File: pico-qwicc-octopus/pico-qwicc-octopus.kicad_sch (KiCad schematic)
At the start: 21 parts, among them U1 RP2040

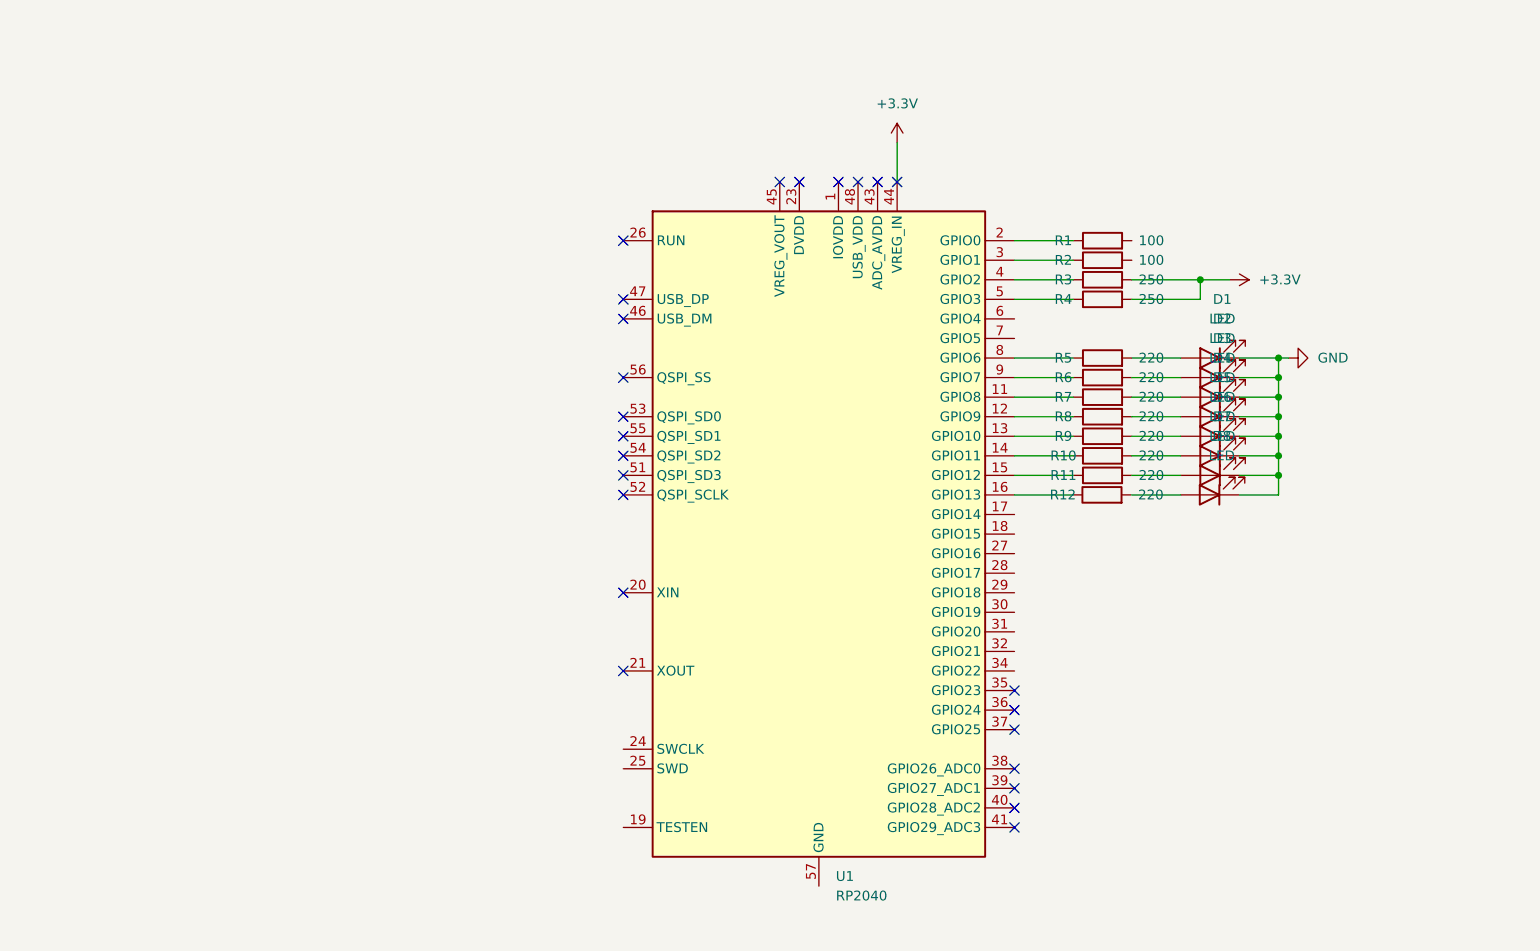
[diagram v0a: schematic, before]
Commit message: Trying to get just the basics working.
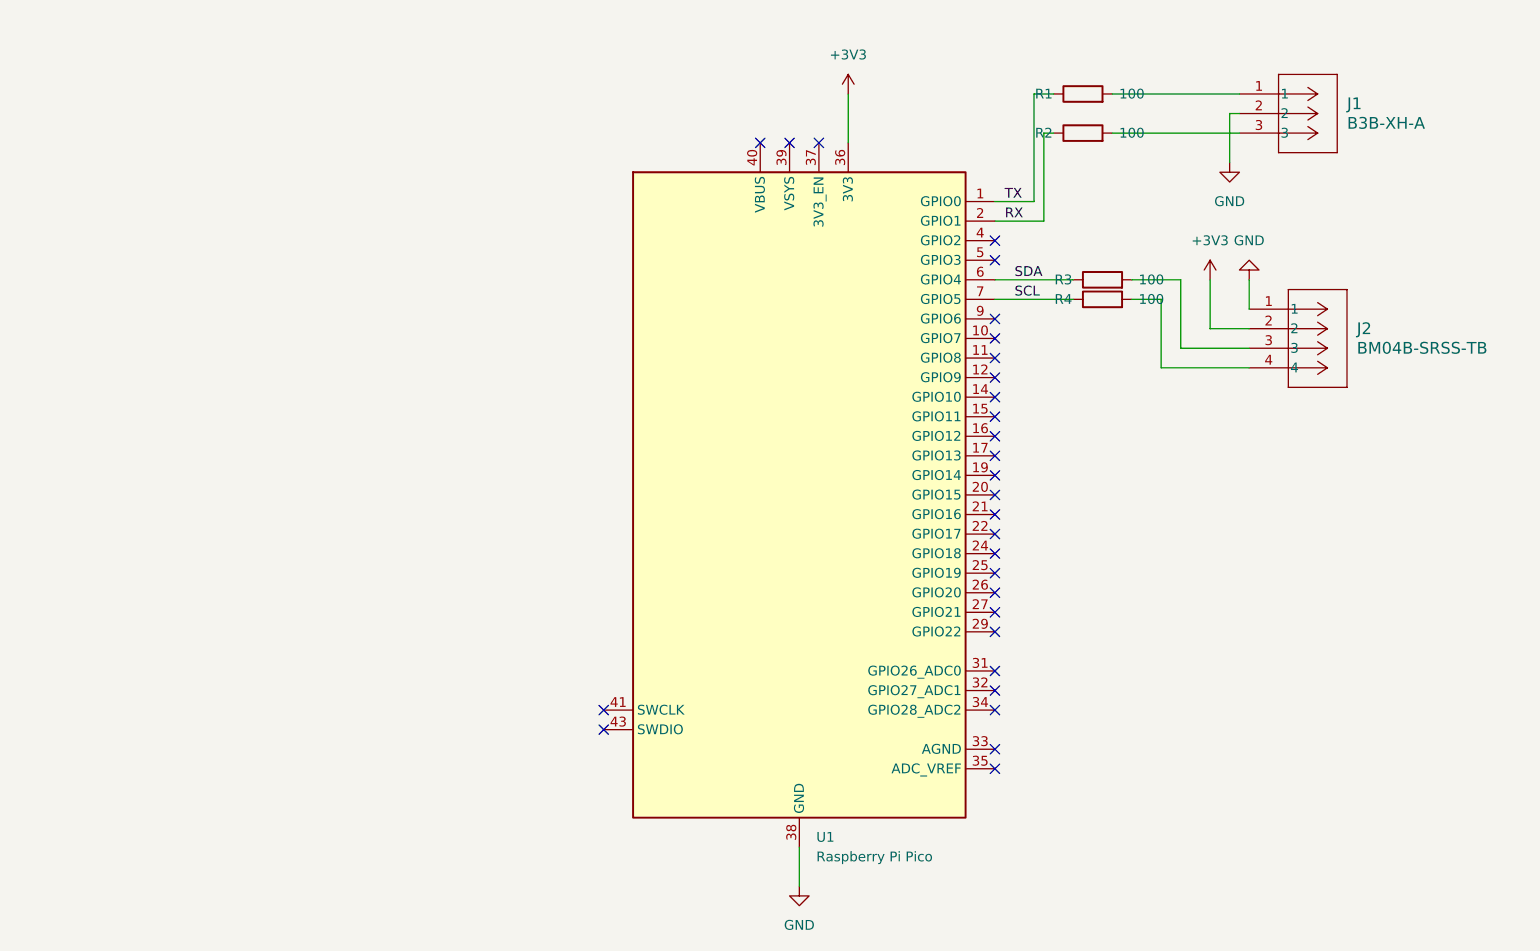
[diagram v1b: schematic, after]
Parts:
- removed D1, D2, D3, D4, D6, D7, D8: LED, LED_SMD:LED_0805_2012Metric, symbol Device:LED
- removed D5: LED, symbol Device:LED
- removed R10, R11, R12, R5, R6, R7, R8, R9: 220, Resistor_SMD:R_0805_2012Metric, symbol Device:R
- removed U1: RP2040, Package_DFN_QFN:QFN-56-1EP_7x7mm_P0.4mm_EP3.2x3.2mm, symbol MCU_RaspberryPi:RP2040
- added J1: B3B-XH-A, CONN_B3B-XH-A_JST, symbol Ivan Hawkes:B3B-XH-A
- added J2: BM04B-SRSS-TB, CONN4_BM04B-SRSS_JST, symbol Ivan Hawkes:BM04B-SRSS-TB
- added U1: Raspberry Pi Pico, Footprint, symbol Ivan Hawkes:Raspberry_Pi_Pico
- R3, R4: value 250 -> 100
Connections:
- net GND: now also J1.2, J2.1, U1.38 (GND)
- net TX: now reaches R1.1
- net TX: now also U1.1 (GPIO0)
- net RX: now reaches R2.1
- net RX: now also U1.2 (GPIO1)
- net SDA: now reaches R3.1
- net SDA: now also U1.6 (GPIO4)
- net SCL: now reaches R4.1
- net SCL: now also U1.7 (GPIO5)
- net at R2.2: now also J1.3
- net at R1.2: now also J1.1
- net +3.3V: no longer names the net of R4.2
- net +3.3V: now also J2.4; no longer R3.2
- new net: J2.3, R3.2
- new net +3V3: J2.2, U1.36 (3V3)
- no-connect marks 24 -> 29
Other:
- moved on the sheet: R1, R2

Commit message: Trying to get a good working symbol for the RPi Pico board.
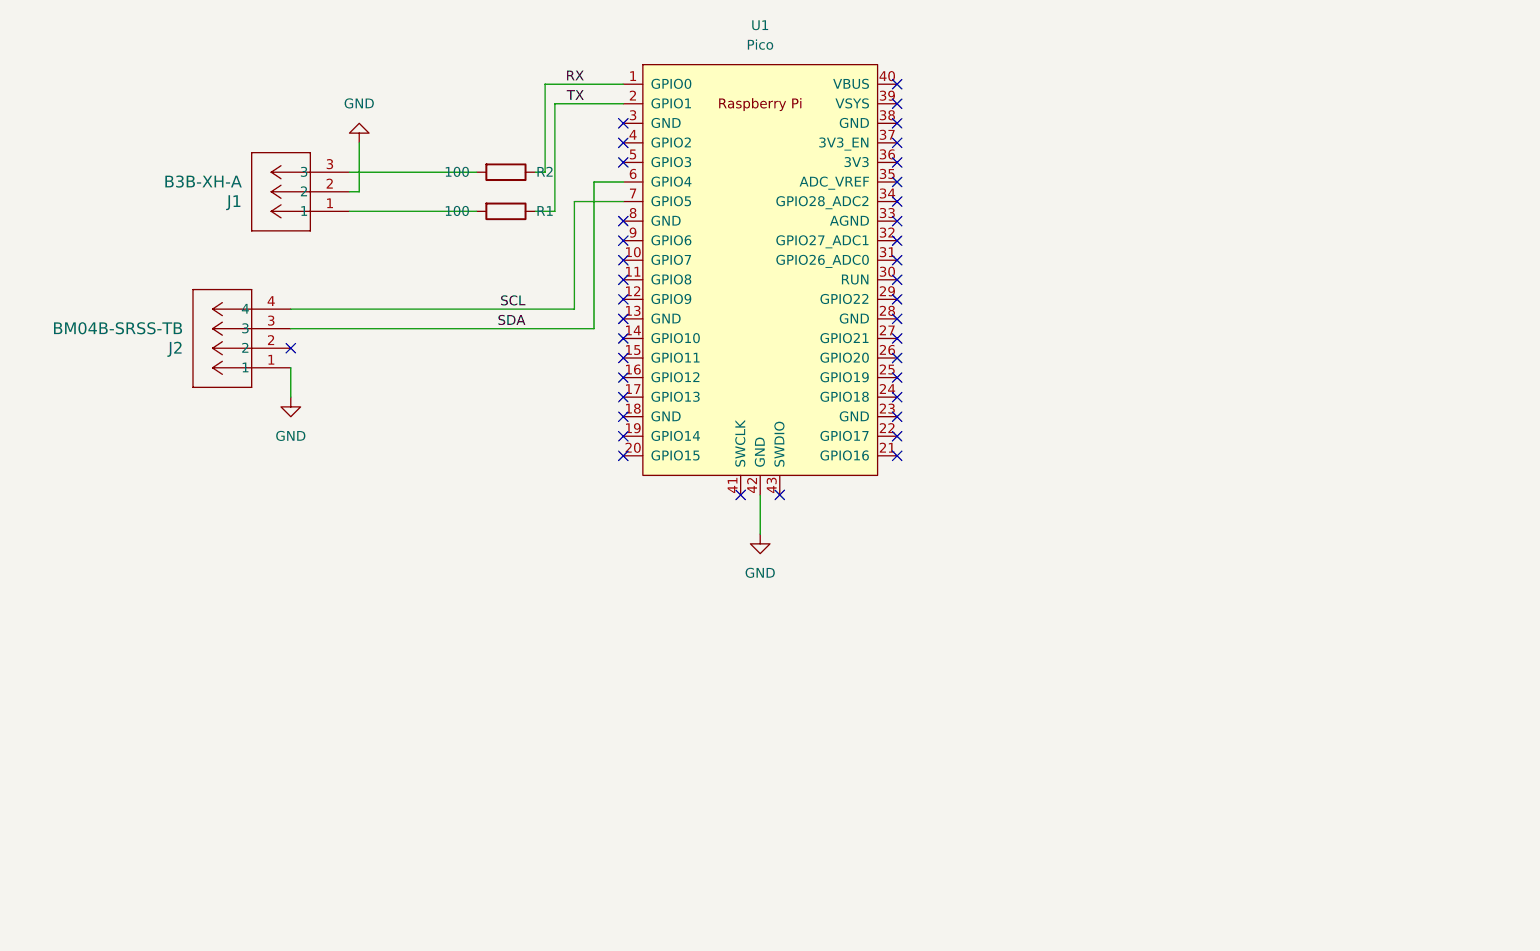
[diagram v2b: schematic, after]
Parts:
- removed R3, R4: 100, Resistor_SMD:R_0805_2012Metric, symbol Device:R
- removed U1: Raspberry Pi Pico, Footprint, symbol Ivan Hawkes:Raspberry_Pi_Pico
- added U1: Pico, RPi_Pico:RPi_Pico_SMD_TH, symbol Ivan Hawkes:Pico
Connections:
- net GND: now also U1.42 (GND)
- net RX: now also U1.1 (GPIO0)
- net SCL: now also J2.4, U1.7 (GPIO5)
- net SDA: now also J2.3, U1.6 (GPIO4)
- net TX: now also U1.2 (GPIO1)
- net +3V3: no longer names the net of J2.2
- no-connect marks 29 -> 39
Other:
- moved on the sheet: J1, J2, R1, R2
